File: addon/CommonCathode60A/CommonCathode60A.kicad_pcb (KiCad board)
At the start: 2 copper layers, 19 parts, among them J101 Conn_02x20_Odd_Even Header, J102 TBL008V-1000-08BE, J103 TBL008V-1000-08BE, K101 EW60-1A3-CL12D04, K102 EW60-1A3-CL12D04, K103 EW60-1A3-CL12D04, K104 EW60-1A3-CL12D04, K105 EW60-1A3-CL12D04, K106 EW60-1A3-CL12D04, K107 EW60-1A3-CL12D04, K108 EW60-1A3-CL12D04

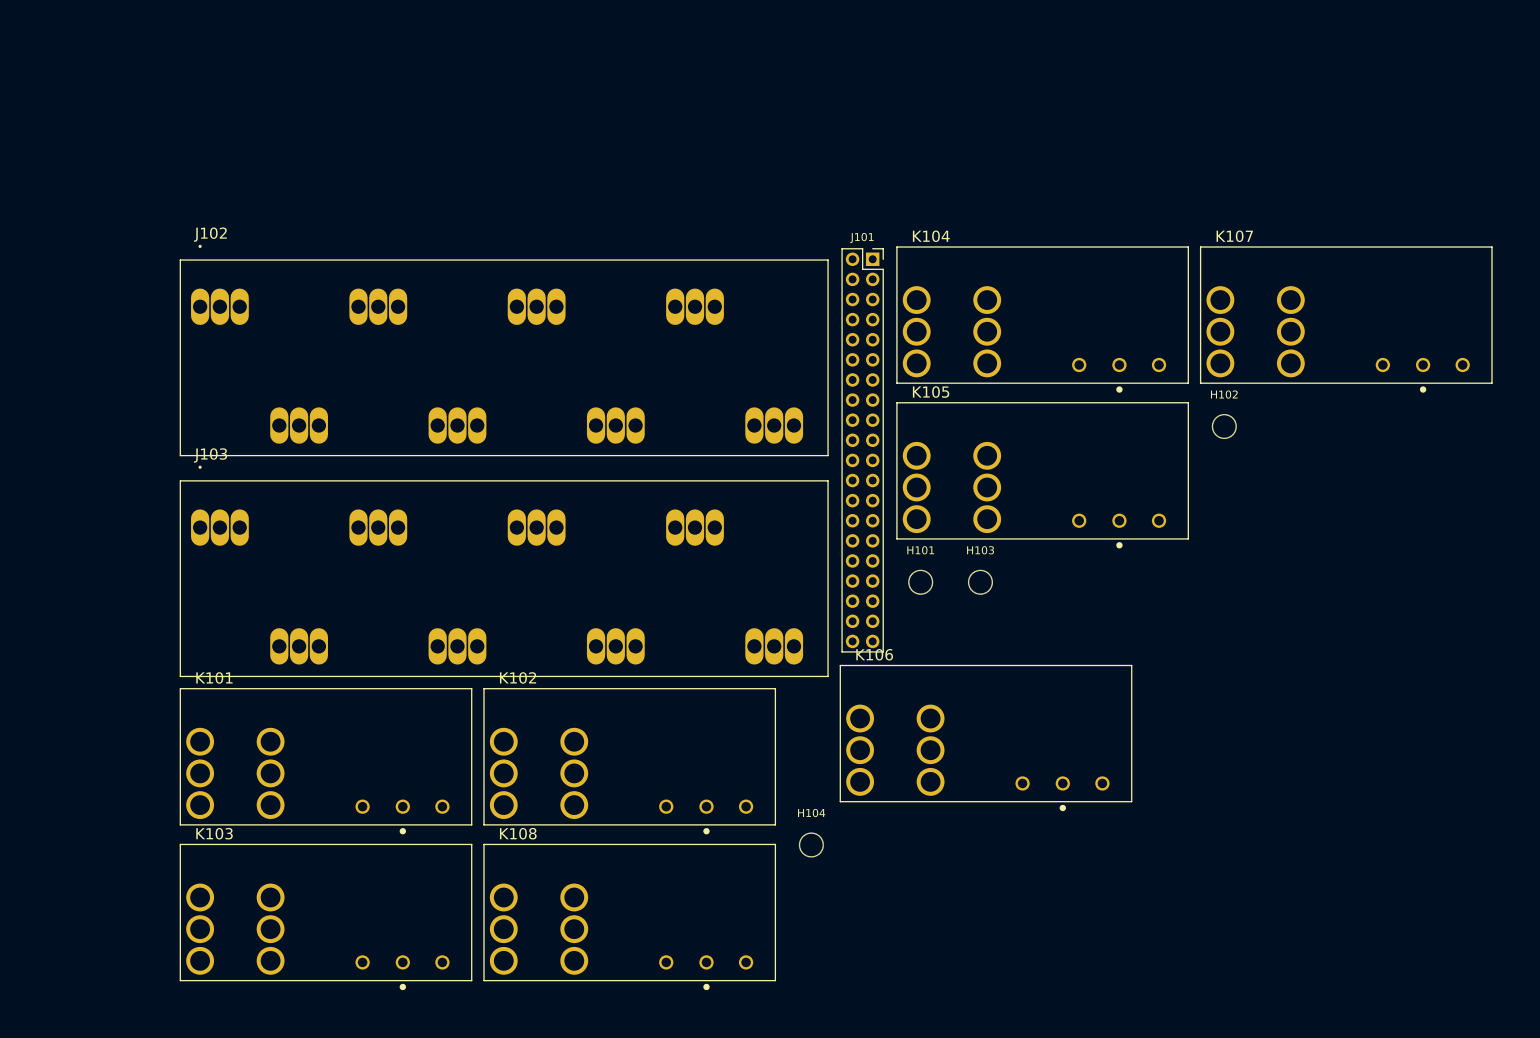
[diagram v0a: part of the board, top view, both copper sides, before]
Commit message: Better 60a board
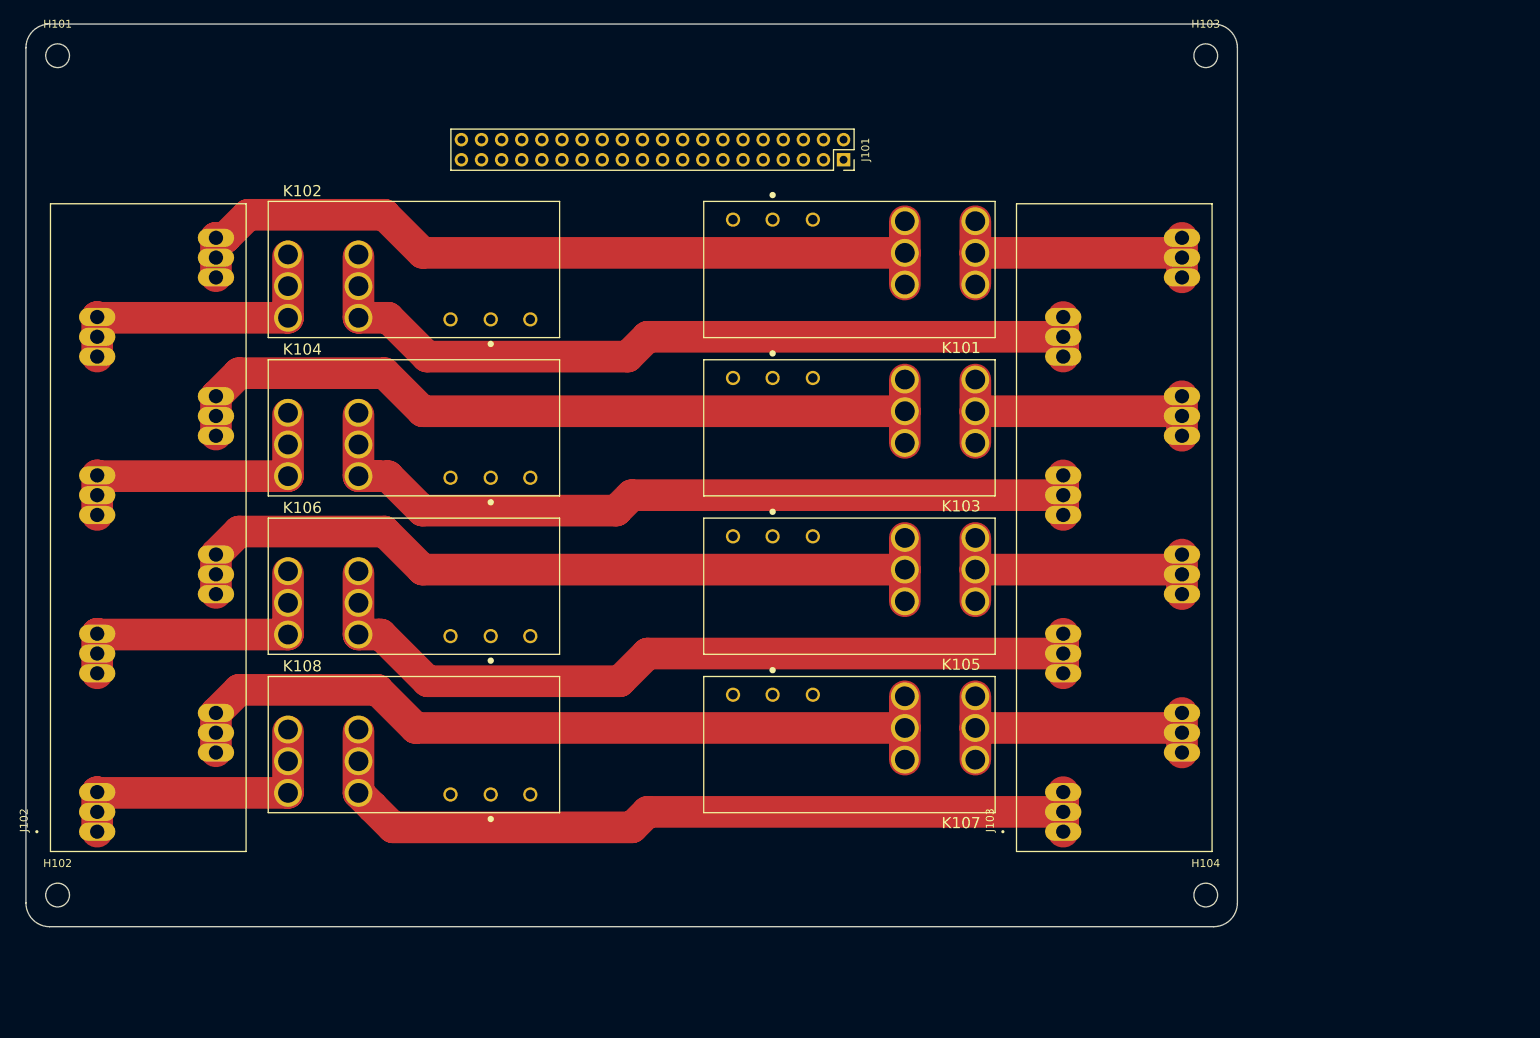
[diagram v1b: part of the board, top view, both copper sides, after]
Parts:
- moved H102 158.8 mm to (54.0, 133.0)
- moved H101 127.7 mm to (54.0, 27.0)
- moved J103 115.6 mm to (181.0, 125.0), turned to 90 degrees
- moved K101 90.3 mm to (154.0, 54.0), turned to 180 degrees
- moved K103 90.1 mm to (154.0, 74.0), turned to 180 degrees
- moved K107 82.9 mm to (154.0, 114.0), turned to 180 degrees
- moved K104 80.7 mm to (99.0, 74.0)
- moved K106 74.6 mm to (99.0, 94.0)
- moved H103 72.3 mm to (199.0, 27.0)
- moved J102 67.6 mm to (59.0, 125.0), turned to 90 degrees
- moved K102 67.3 mm to (99.0, 54.0)
- moved H104 50.2 mm to (199.0, 133.0)
- moved K108 34.5 mm to (99.0, 114.0)
- moved K105 28.4 mm to (154.0, 94.0), turned to 180 degrees
- moved J101 13.1 mm to (153.3, 40.1), turned to 270 degrees
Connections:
- net /K2_COIL_ON renamed /K4_COIL_ON
- J101 pad 13: /K2_COIL_OFF -> /K4_COIL_OFF
- J101 pad 14: /K2_COIL_OFF -> /K4_COIL_OFF
- K104 pad A2: /K2_COIL_OFF -> /K4_COIL_OFF
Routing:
- net /K3_OUT: track 0.00 -> 105.7 mm
- net /K1_OUT: track 0.00 -> 104.8 mm
- net /K2_OUT: track 0.00 -> 104.4 mm
- net /K4_OUT: track 0.00 -> 104.4 mm
- net /K8_IN: track 0.00 -> 103.0 mm
- net /K7_IN: track 0.00 -> 103.0 mm
- net /K6_IN: track 0.00 -> 103.0 mm
- net /K5_IN: track 0.00 -> 103.0 mm
- net /K5_OUT: track 0.00 -> 39.3 mm
- net /K8_OUT: track 0.00 -> 39.3 mm
- net /K7_OUT: track 0.00 -> 39.3 mm
- net /K6_OUT: track 0.00 -> 39.3 mm
- net /K1_IN: track 0.00 -> 36.9 mm
- net /K4_IN: track 0.00 -> 36.9 mm
- net /K3_IN: track 0.00 -> 36.9 mm
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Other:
- board outline added: 153 x 114 mm
- net class 30A Up to 230V AC added: clearance 1.25, trace_width 4, via_dia 9, via_drill 7
- net class 60A Up to 230V AC added: clearance 1.25, trace_width 8, via_dia 9, via_drill 7
- net class Default: clearance 0.2 -> 0.25; via_drill 0.4 -> 0.5
- rule trace_clearance: 0.2 -> 0.25
